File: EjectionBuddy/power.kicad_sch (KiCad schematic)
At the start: 8 parts, among them U3 LP5912-3.3DRV, U4 LM66200DRLR, U5 GenericBuck_5V

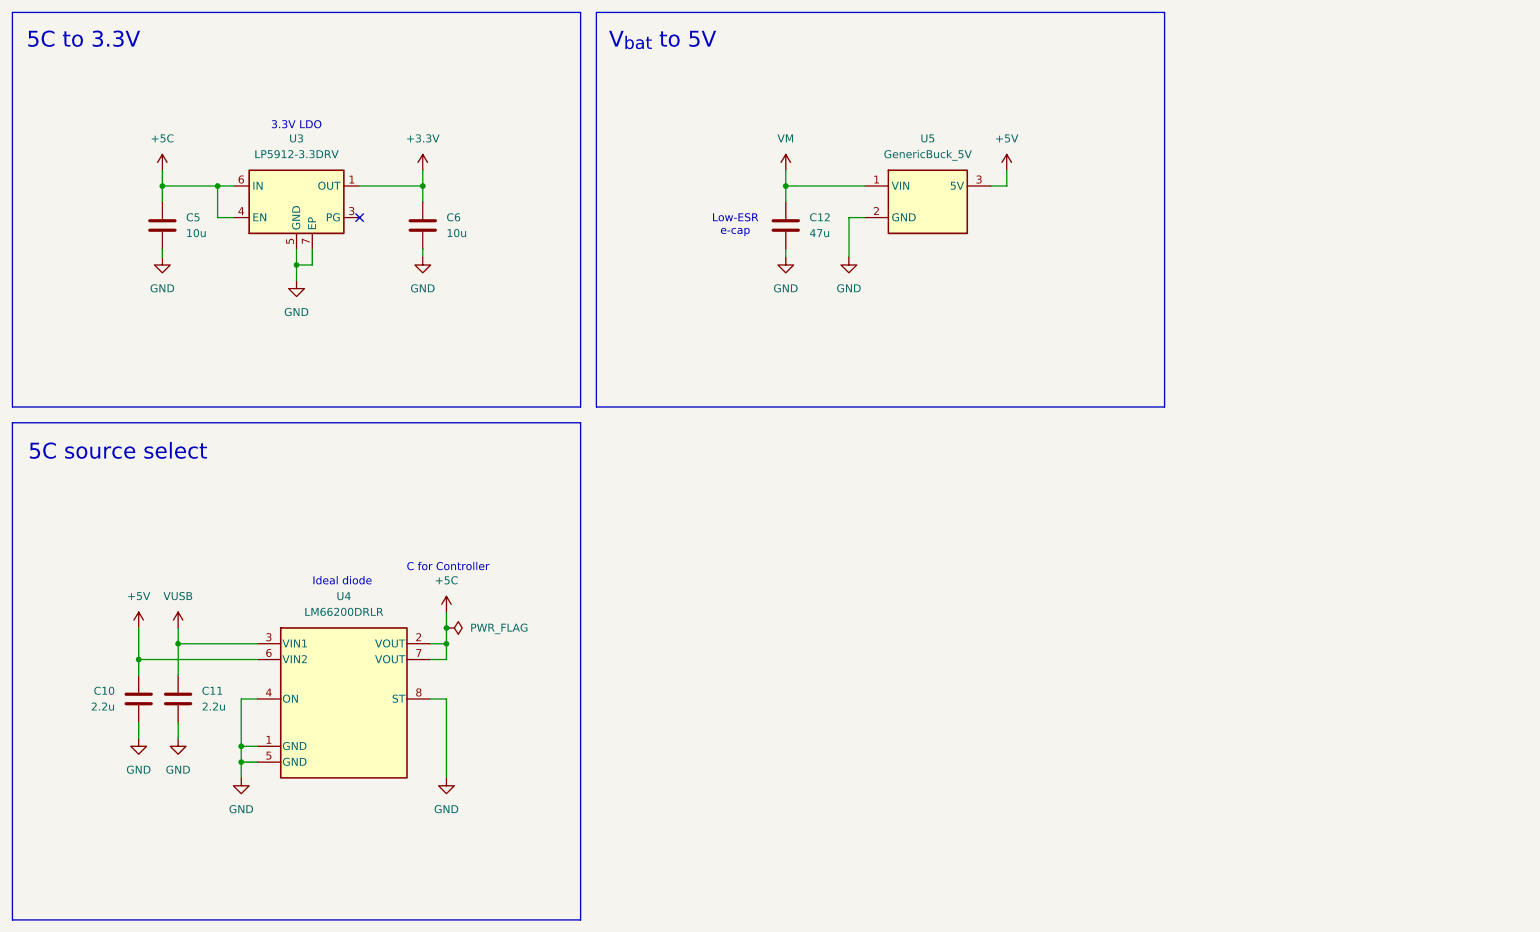
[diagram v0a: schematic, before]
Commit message: Finished! QR and instruction pending
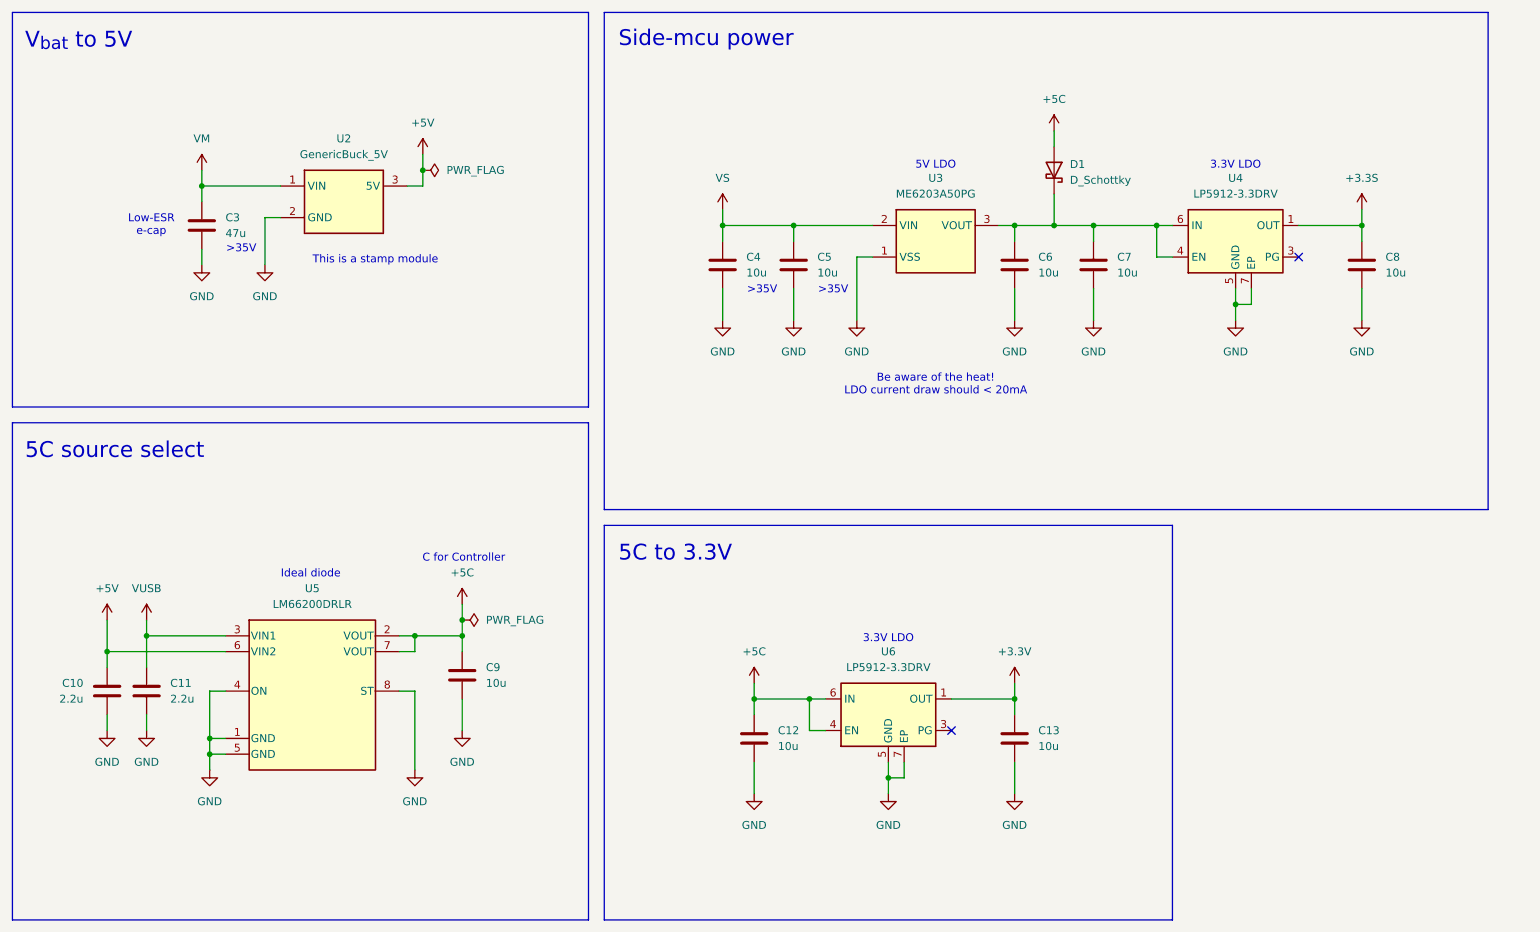
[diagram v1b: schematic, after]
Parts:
- added C4, C5, C6, C7, C8, C9: 10u, Capacitor_SMD:C_0603_1608Metric, symbol Device:C
- added D1: D_Schottky, Diode_SMD:D_SOD-523, symbol Device:D_Schottky
- added U3: ME6203A50PG, Package_TO_SOT_SMD:SOT-89-3, symbol ME6203:ME6203A50PG
- added U4: LP5912-3.3DRV, Package_SON:WSON-6-1EP_2x2mm_P0.65mm_EP1x1.6mm_ThermalVias, symbol Regulator_Linear:LP5912-3.3DRV
- C3: renamed from C12; footprint Capacitor_SMD:C_0603_1608Metric -> Capacitor_SMD:CP_Elec_5x4.5
- U2: renamed from U5; footprint (none) -> MP4462BuckModule_TaoBao_20x17:MP4462BuckModule_TaoBao_20x17
- U5: renamed from U4; footprint SOT-5X3_DRL_TEX -> Package_TO_SOT_SMD:SOT-583-8
- renumbered C5 to C12, C6 to C13, U3 to U6
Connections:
- net +5C: now also C9.1, D1.2 (A)
- net GND: now also C4.2, C5.2, C6.2, C7.2, C8.2, C9.2, U3.1 (VSS), U4.5 (GND), U4.7 (EP)
- new net: C6.1, C7.1, D1.1 (K), U3.3 (VOUT), U4.4 (EN), U4.6 (IN)
- new net +3.3S: C8.1, U4.1 (OUT)
- new net VS: C4.1, C5.1, U3.2 (VIN)
- no-connect marks 1 -> 2
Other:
- note added: "5V LDO"
- note added: ">35V"
- note added: "Be aware of the heat! LDO current draw should < 20mA"
- note added: "Side-mcu power"
- note added: "This is a stamp module"
- moved on the sheet: C10, C11, C12, C13, C3, U2, U5, U6

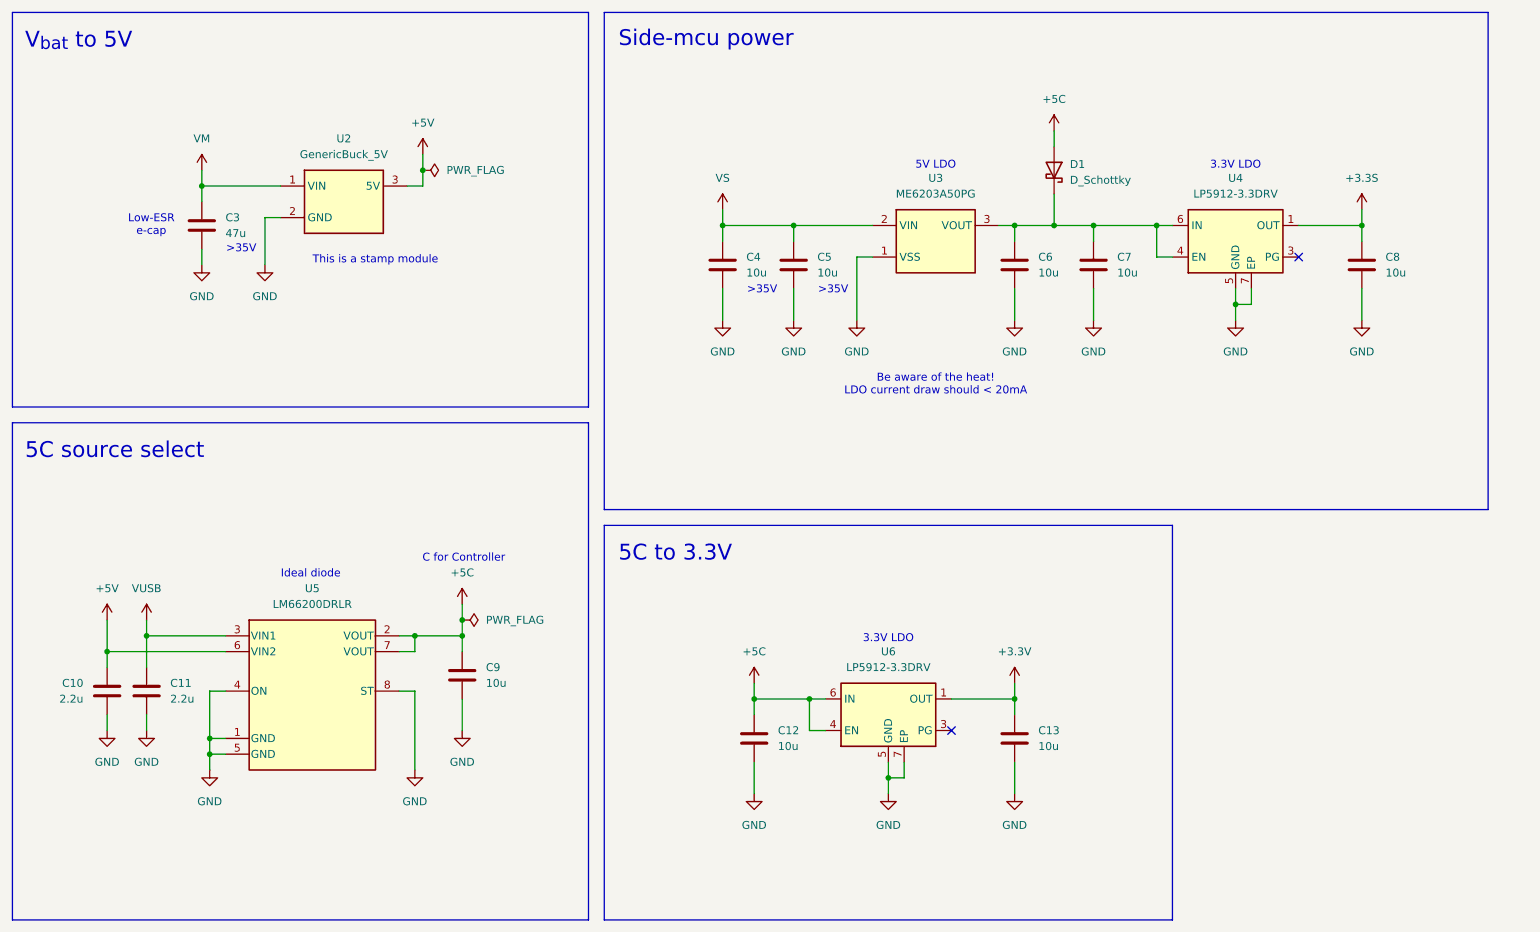
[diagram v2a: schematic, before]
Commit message: Prodection version hw1.0 finished, with tidy-ups and bug-fixes
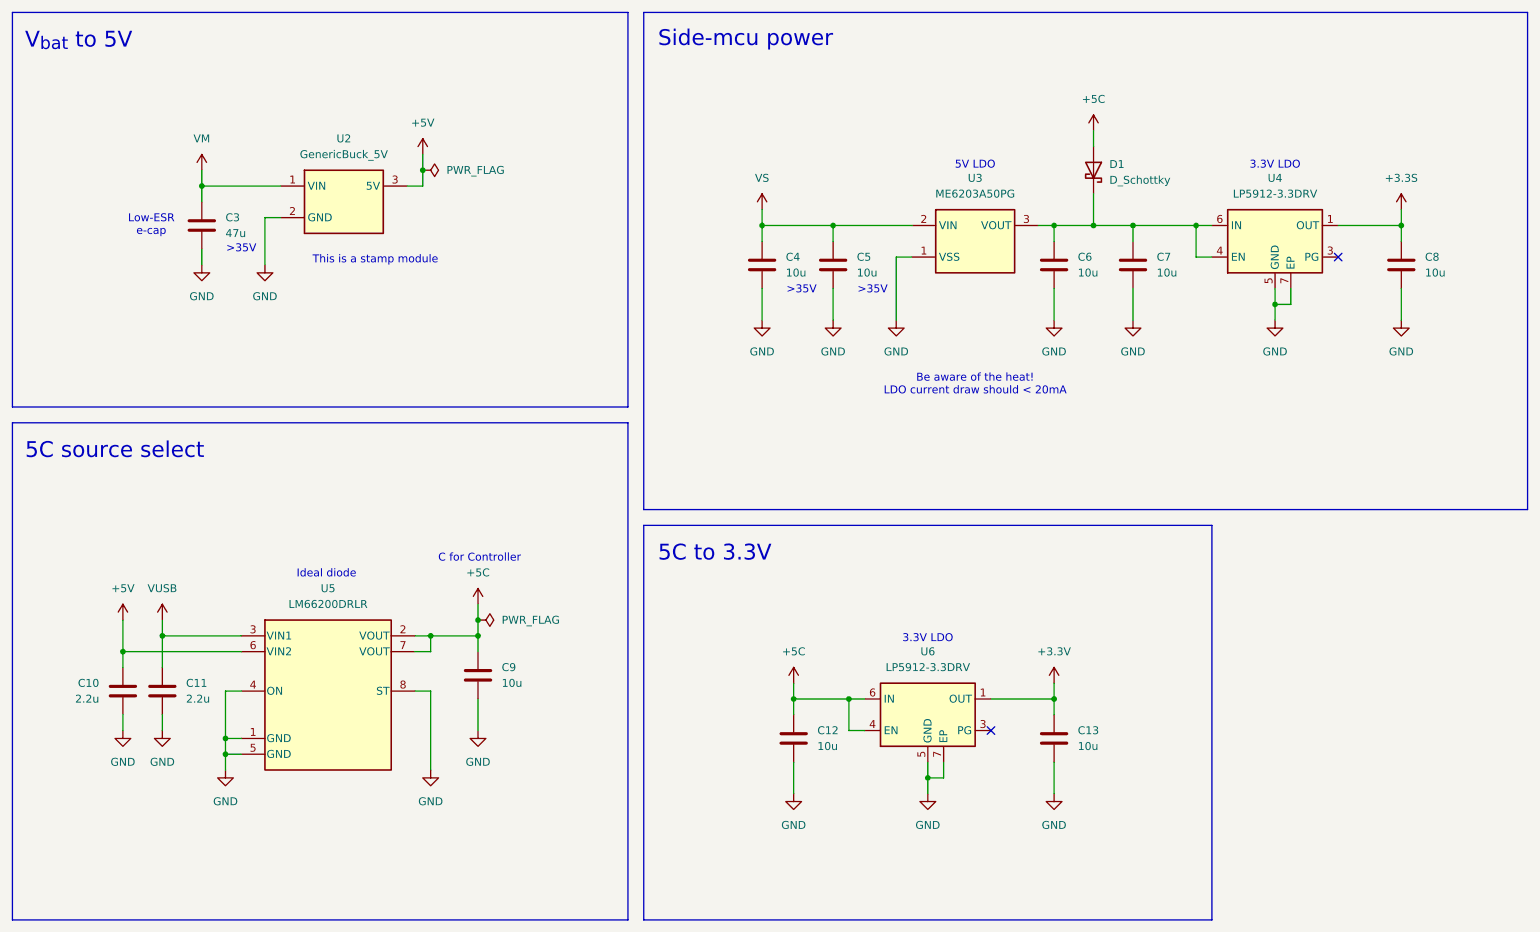
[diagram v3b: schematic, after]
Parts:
- C3: footprint Capacitor_SMD:CP_Elec_5x4.5 -> Capacitor_SMD:CP_Elec_6.3x5.8
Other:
- moved on the sheet: C10, C11, C12, C13, C4, C5, C6, C7, C8, C9, D1, U3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
